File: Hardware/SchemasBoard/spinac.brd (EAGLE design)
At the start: 41.5 x 26.9 mm, 29 parts, among them IC1 LNK304, IC3 MC33269ST-3.3T3, IC4 DS1820, K1 FRS1B, T1 BC846

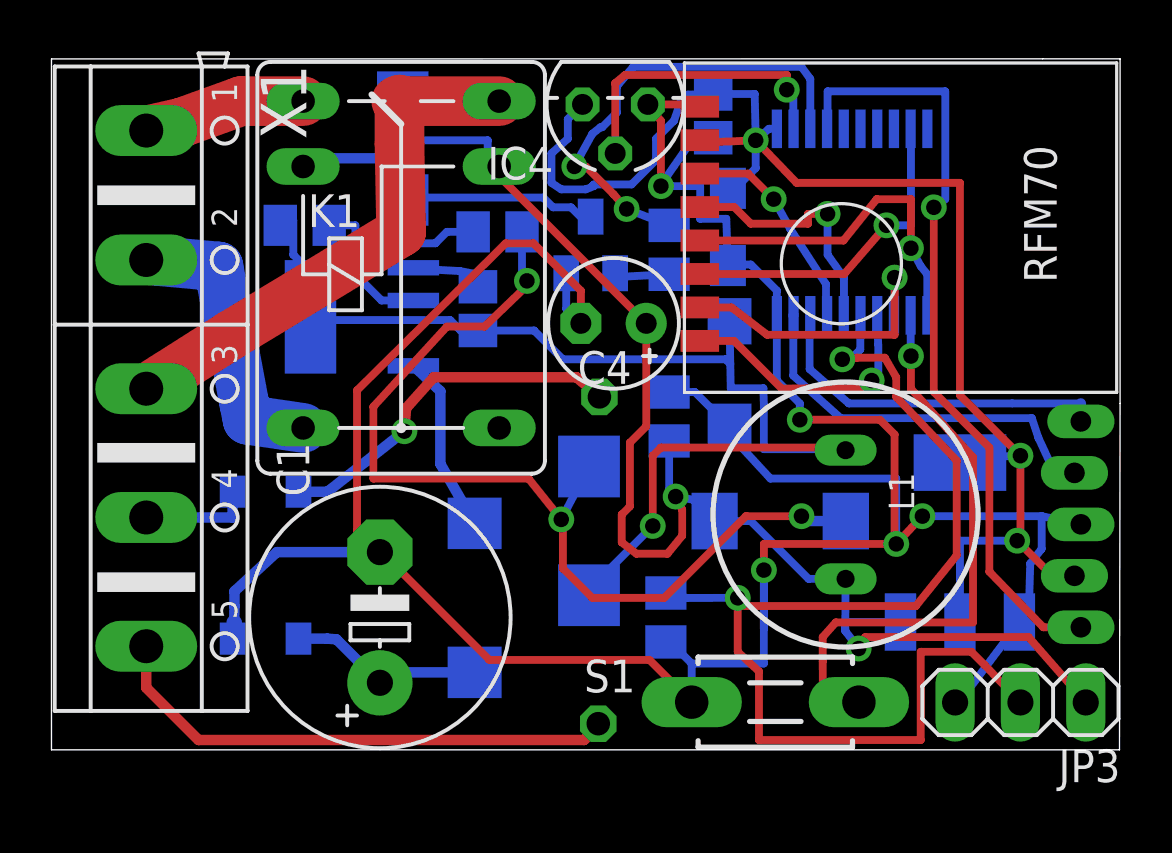
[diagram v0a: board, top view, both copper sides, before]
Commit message: z
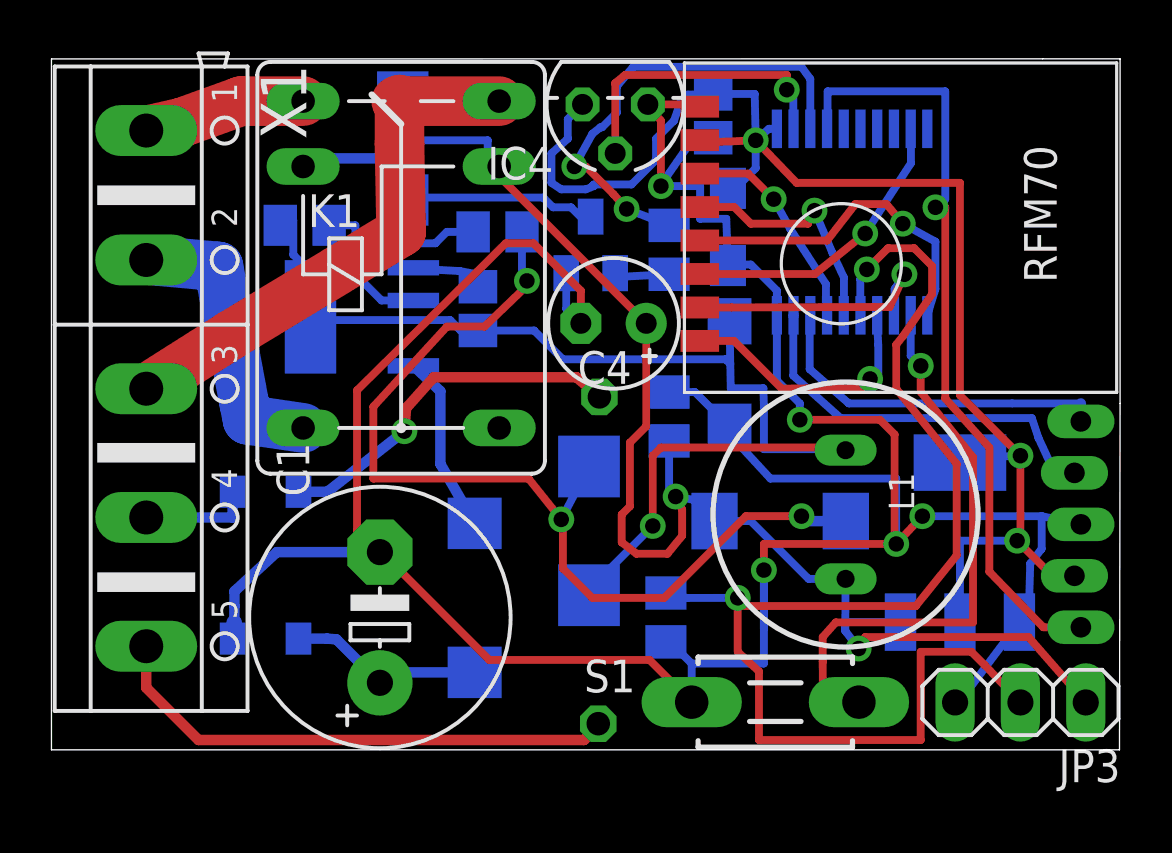
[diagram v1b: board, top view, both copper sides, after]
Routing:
- net N$32: track 45.1 -> 50.1 mm
- net N$23: track 12.8 -> 11.6 mm
- net N$12: track 11.6 -> 10.5 mm
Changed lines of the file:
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@@
 <contactref element="U$2" pad="13"/>
 <wire x1="25.197" y1="17.192" x2="26.4325" y2="17.192" width="0.3048" layer="1"/>
-<wire x1="26.4325" y1="17.192" x2="27.813" y2="16.129" width="0.3048" layer="1"/>
-<wire x1="27.813" y1="16.129" x2="32.766" y2="16.129" width="0.3048" layer="1"/>
-<wire x1="32.766" y1="16.129" x2="32.766" y2="18.3515" width="0.3048" layer="1"/>
-<via x="32.766" y="18.3515" extent="1-16" drill="0.6"/>
-<wire x1="32.766" y1="18.3515" x2="32.766" y2="16.9115" width="0.3048" layer="16"/>
+<wire x1="26.4325" y1="17.192" x2="31.9405" y2="17.2085" width="0.3048" layer="1"/>
+<wire x1="31.9405" y1="17.2085" x2="32.5755" y2="17.2085" width="0.3048" layer="1"/>
+<wire x1="32.5755" y1="17.2085" x2="33.147" y2="18.4785" width="0.3048" layer="1"/>
+<via x="33.147" y="18.4785" extent="1-16" drill="0.6"/>
 <wire x1="32.766" y1="16.9115" x2="32.74" y2="16.8855" width="0.3048" layer="16"/>
+<wire x1="32.766" y1="16.9115" x2="32.766" y2="17.907" width="0.3048" layer="16"/>
+<wire x1="32.766" y1="17.907" x2="33.147" y2="18.4785" width="0.3048" layer="16"/>
 </signal>
 <signal name="N$18">
@@
 <wire x1="27.178" y1="20.447" x2="29.4005" y2="20.447" width="0.3048" layer="1"/>
 <wire x1="29.4005" y1="20.447" x2="29.4005" y2="20.828" width="0.3048" layer="1"/>
-<wire x1="29.4005" y1="20.828" x2="30.1625" y2="20.828" width="0.3048" layer="1"/>
-<via x="30.1625" y="20.828" extent="1-16" drill="0.6"/>
-<wire x1="30.1625" y1="20.828" x2="30.1625" y2="19.2405" width="0.3048" layer="16"/>
-<wire x1="30.1625" y1="19.2405" x2="30.7975" y2="18.3515" width="0.3048" layer="16"/>
+<wire x1="29.4005" y1="20.828" x2="29.6545" y2="20.955" width="0.3048" layer="1"/>
+<via x="29.6545" y="20.955" extent="1-16" drill="0.6"/>
+<wire x1="29.6545" y1="20.955" x2="30.353" y2="19.304" width="0.3048" layer="16"/>
+<wire x1="30.353" y1="19.304" x2="30.7975" y2="18.3515" width="0.3048" layer="16"/>
 <wire x1="30.7975" y1="18.3515" x2="30.7975" y2="16.893" width="0.3048" layer="16"/>
 <wire x1="30.7975" y1="16.893" x2="30.79" y2="16.8855" width="0.3048" layer="16"/>
@@
 <wire x1="26.526" y1="15.892" x2="28.3845" y2="14.0335" width="0.3048" layer="1"/>
 <wire x1="28.3845" y1="14.0335" x2="31.877" y2="14.097" width="0.3048" layer="1"/>
-<wire x1="31.877" y1="14.097" x2="31.877" y2="14.351" width="0.3048" layer="1"/>
-<via x="31.877" y="14.351" extent="1-16" drill="0.6"/>
-<wire x1="31.877" y1="14.351" x2="32.131" y2="14.605" width="0.3048" layer="16"/>
+<wire x1="31.877" y1="14.097" x2="31.8135" y2="14.4145" width="0.3048" layer="1"/>
+<via x="31.8135" y="14.4145" extent="1-16" drill="0.6"/>
+<wire x1="31.8135" y1="14.4145" x2="32.131" y2="14.605" width="0.3048" layer="16"/>
 <wire x1="32.131" y1="14.605" x2="32.131" y2="15.748" width="0.3048" layer="16"/>
 <wire x1="32.131" y1="15.748" x2="32.0675" y2="16.863" width="0.3048" layer="16"/>
@@
 <contactref element="U$2" pad="11"/>
 <contactref element="U$1" pad="SCK"/>
-<wire x1="25.197" y1="19.792" x2="30.7775" y2="19.792" width="0.3048" layer="1"/>
-<wire x1="30.7775" y1="19.792" x2="32.0675" y2="21.3995" width="0.3048" layer="1"/>
-<wire x1="32.0675" y1="21.3995" x2="33.401" y2="21.3995" width="0.3048" layer="1"/>
-<wire x1="33.401" y1="21.3995" x2="33.401" y2="19.4945" width="0.3048" layer="1"/>
-<via x="33.401" y="19.4945" extent="1-16" drill="0.6"/>
-<wire x1="33.401" y1="19.4945" x2="33.782" y2="18.796" width="0.3048" layer="16"/>
-<wire x1="33.782" y1="18.796" x2="34.036" y2="18.4785" width="0.3048" layer="16"/>
-<wire x1="34.036" y1="18.4785" x2="34.036" y2="16.8895" width="0.3048" layer="16"/>
+<wire x1="25.197" y1="19.792" x2="30.1425" y2="19.792" width="0.3048" layer="1"/>
+<wire x1="30.1425" y1="19.792" x2="31.242" y2="21.209" width="0.3048" layer="1"/>
+<wire x1="31.242" y1="21.209" x2="32.4485" y2="21.209" width="0.3048" layer="1"/>
+<wire x1="32.4485" y1="21.209" x2="33.0835" y2="20.447" width="0.3048" layer="1"/>
+<via x="33.0835" y="20.447" extent="1-16" drill="0.6"/>
+<wire x1="33.0835" y1="20.447" x2="34.3535" y2="19.7485" width="0.3048" layer="16"/>
+<wire x1="34.3535" y1="19.7485" x2="34.3535" y2="17.907" width="0.3048" layer="16"/>
+<wire x1="34.3535" y1="17.907" x2="34.036" y2="16.8895" width="0.3048" layer="16"/>
 <wire x1="34.036" y1="16.8895" x2="34.04" y2="16.8855" width="0.3048" layer="16"/>
 </signal>
@@
 <contactref element="U$2" pad="9"/>
 <contactref element="U$1" pad="MOSI"/>
-<wire x1="25.197" y1="18.492" x2="30.811" y2="18.492" width="0.3048" layer="1"/>
-<wire x1="30.811" y1="18.492" x2="32.4485" y2="20.3835" width="0.3048" layer="1"/>
-<via x="32.4485" y="20.3835" extent="1-16" drill="0.6"/>
-<wire x1="32.4485" y1="20.3835" x2="33.401" y2="20.3835" width="0.3048" layer="16"/>
-<wire x1="33.401" y1="20.3835" x2="33.401" y2="24.083" width="0.3048" layer="16"/>
+<wire x1="25.197" y1="18.492" x2="29.668" y2="18.492" width="0.3048" layer="1"/>
+<wire x1="29.668" y1="18.492" x2="31.623" y2="20.066" width="0.3048" layer="1"/>
+<via x="31.623" y="20.066" extent="1-16" drill="0.6"/>
+<wire x1="31.623" y1="20.066" x2="33.401" y2="22.7965" width="0.3048" layer="16"/>
+<wire x1="33.401" y1="22.7965" x2="33.401" y2="24.083" width="0.3048" layer="16"/>
 <wire x1="33.401" y1="24.083" x2="33.39" y2="24.1355" width="0.3048" layer="16"/>
 </signal>
@@
 <wire x1="30.1625" y1="25.5905" x2="34.7345" y2="25.5905" width="0.3048" layer="16"/>
 <wire x1="34.7345" y1="25.5905" x2="34.7345" y2="21.3995" width="0.3048" layer="16"/>
-<wire x1="34.7345" y1="21.3995" x2="34.29" y2="21.082" width="0.3048" layer="16"/>
-<via x="34.29" y="21.082" extent="1-16" drill="0.6"/>
-<wire x1="34.29" y1="21.082" x2="34.29" y2="13.9065" width="0.3048" layer="1"/>
-<wire x1="34.29" y1="13.9065" x2="36.449" y2="11.7475" width="0.3048" layer="1"/>
+<wire x1="34.7345" y1="21.3995" x2="34.3535" y2="21.082" width="0.3048" layer="16"/>
+<via x="34.3535" y="21.082" extent="1-16" drill="0.6"/>
+<wire x1="34.7345" y1="13.6525" x2="36.449" y2="11.7475" width="0.3048" layer="1"/>
 <wire x1="36.449" y1="11.7475" x2="36.449" y2="6.9215" width="0.3048" layer="1"/>
 <wire x1="36.449" y1="6.9215" x2="38.544" y2="4.7625" width="0.3048" layer="1"/>
 <wire x1="38.544" y1="4.7625" x2="40.005" y2="4.763" width="0.3048" layer="1"/>
+<wire x1="34.3535" y1="21.082" x2="34.7345" y2="21.082" width="0.3048" layer="1"/>
+<wire x1="34.7345" y1="21.082" x2="34.7345" y2="13.6525" width="0.3048" layer="1"/>
 </signal>
 <signal name="N$14">
@@
 <contactref element="U$2" pad="15"/>
 <contactref element="JP3" pad="2"/>
-<wire x1="32.8295" y1="14.478" x2="32.385" y2="15.24" width="0.3048" layer="1"/>
-<wire x1="32.385" y1="15.24" x2="31.3055" y2="15.24" width="0.3048" layer="1"/>
-<wire x1="31.3055" y1="15.24" x2="30.734" y2="15.1765" width="0.3048" layer="1"/>
-<via x="30.734" y="15.1765" extent="1-16" drill="0.6"/>
-<wire x1="30.734" y1="15.1765" x2="31.115" y2="15.24" width="0.3048" layer="16"/>
-<wire x1="31.115" y1="15.24" x2="31.4325" y2="15.5575" width="0.3048" layer="16"/>
-<wire x1="31.4325" y1="15.5575" x2="31.4325" y2="16.878" width="0.3048" layer="16"/>
+<via x="31.6865" y="18.669" extent="1-16" drill="0.6"/>
 <wire x1="31.4325" y1="16.878" x2="31.44" y2="16.8855" width="0.3048" layer="16"/>
-<wire x1="32.8295" y1="14.478" x2="32.8295" y2="13.716" width="0.3048" layer="1"/>
-<wire x1="32.8295" y1="13.716" x2="35.179" y2="11.2395" width="0.3048" layer="1"/>
+<wire x1="32.8295" y1="14.0335" x2="35.179" y2="11.1125" width="0.3048" layer="1"/>
 <wire x1="27.4955" y1="3.048" x2="27.4955" y2="0.381" width="0.3048" layer="1"/>
 <wire x1="27.4955" y1="0.381" x2="33.782" y2="0.381" width="0.3048" layer="1"/>
@@
 <wire x1="27.4955" y1="3.048" x2="26.67" y2="3.81" width="0.3048" layer="1"/>
 <wire x1="26.67" y1="3.81" x2="26.67" y2="5.588" width="0.3048" layer="1"/>
-<wire x1="35.179" y1="11.2395" x2="35.179" y2="7.5565" width="0.3048" layer="1"/>
+<wire x1="35.179" y1="11.1125" x2="35.179" y2="7.5565" width="0.3048" layer="1"/>
 <wire x1="35.179" y1="7.5565" x2="33.5915" y2="5.588" width="0.3048" layer="1"/>
 <wire x1="33.5915" y1="5.588" x2="26.67" y2="5.588" width="0.3048" layer="1"/>
 <wire x1="26.67" y1="5.588" x2="26.67" y2="5.9055" width="0.3048" layer="1"/>
+<wire x1="31.4325" y1="16.878" x2="31.4325" y2="18.288" width="0.3048" layer="16"/>
+<wire x1="31.4325" y1="18.288" x2="31.6865" y2="18.669" width="0.3048" layer="16"/>
+<wire x1="32.8295" y1="14.0335" x2="32.8295" y2="15.748" width="0.3048" layer="1"/>
+<wire x1="32.8295" y1="15.748" x2="33.0835" y2="16.0655" width="0.3048" layer="1"/>
+<wire x1="33.0835" y1="16.0655" x2="34.2265" y2="17.7165" width="0.3048" layer="1"/>
+<wire x1="34.2265" y1="17.7165" x2="34.2265" y2="18.796" width="0.3048" layer="1"/>
+<wire x1="34.2265" y1="18.796" x2="33.528" y2="19.4945" width="0.3048" layer="1"/>
+<wire x1="33.528" y1="19.4945" x2="32.512" y2="19.4945" width="0.3048" layer="1"/>
+<wire x1="32.512" y1="19.4945" x2="31.6865" y2="18.669" width="0.3048" layer="1"/>
 </signal>
 <signal name="N$35">
@@
 <contactref element="U$2" pad="12"/>
 <wire x1="33.39" y1="16.8855" x2="33.39" y2="15.3145" width="0.3048" layer="16"/>
-<wire x1="33.39" y1="15.3145" x2="33.401" y2="15.3035" width="0.3048" layer="16"/>
-<via x="33.401" y="15.3035" extent="1-16" drill="0.6"/>
-<wire x1="33.401" y1="15.3035" x2="33.401" y2="14.0335" width="0.3048" layer="1"/>
-<wire x1="33.401" y1="14.0335" x2="35.814" y2="11.3665" width="0.3048" layer="1"/>
+<wire x1="33.39" y1="15.3145" x2="33.782" y2="14.9225" width="0.3048" layer="16"/>
+<via x="33.782" y="14.9225" extent="1-16" drill="0.6"/>
+<wire x1="33.782" y1="14.9225" x2="33.782" y2="13.9065" width="0.3048" layer="1"/>
+<wire x1="33.782" y1="13.9065" x2="35.814" y2="11.3665" width="0.3048" layer="1"/>
 <wire x1="31.3805" y1="1.853" x2="29.9835" y2="1.8935" width="0.3048" layer="1"/>
 <wire x1="29.9835" y1="1.8935" x2="29.972" y2="3.429" width="0.3048" layer="1"/>
